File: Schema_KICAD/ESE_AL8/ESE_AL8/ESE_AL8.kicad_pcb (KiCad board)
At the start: 4 copper layers, 54 x 57 mm, 85 parts, among them IC1 MP1475SGJ-P, J1 CB1, J2 CB2, J3 LIDAR, J4 Moteur1, J5 Moteur2, J6 Batterie, J7 Conn_ST_STDC14, J8 ECRAN, SW1 SW_c/s, SW2 ON/OFF, U1 ADXL343, U2 BUxxSD5, U3 STM32G431CBUx, U4 ZXBM5210-SP, U5 ZXBM5210-SP, Y1 16MHz

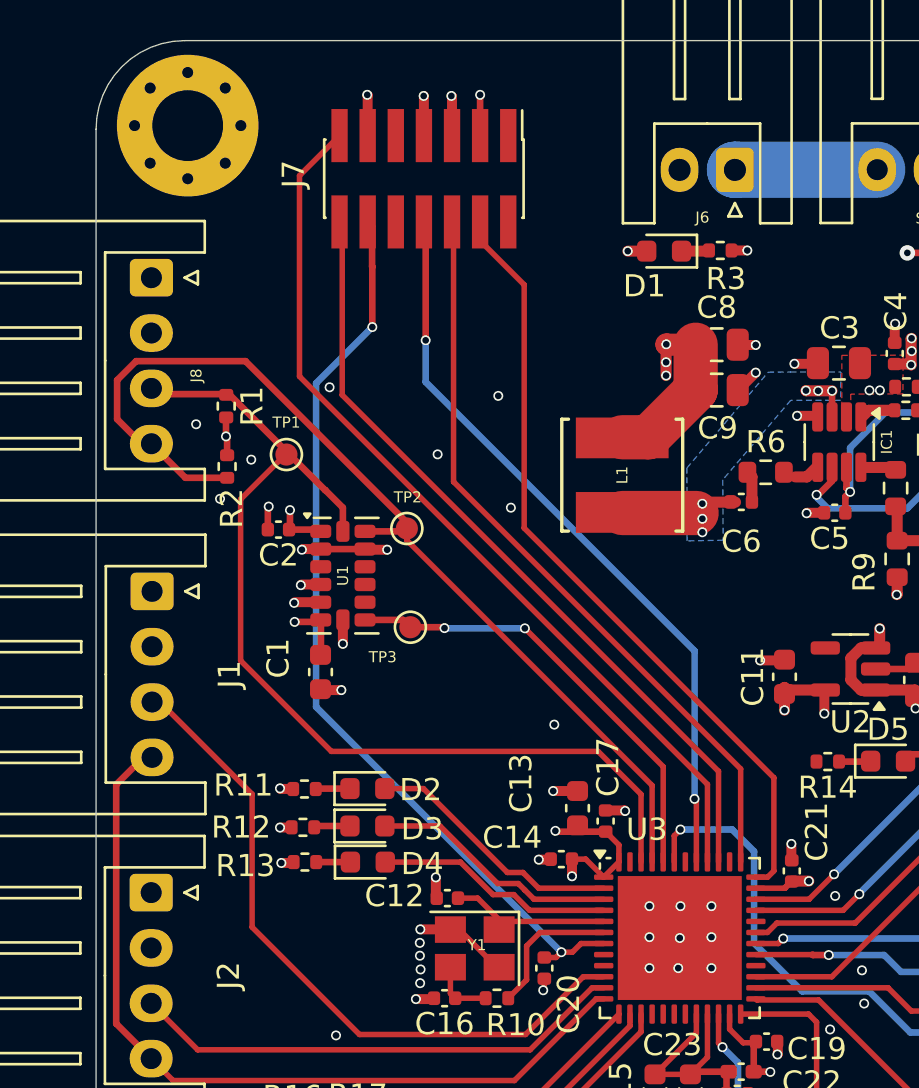
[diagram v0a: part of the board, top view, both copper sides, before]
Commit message: Commit midif pcb 23/10 0816
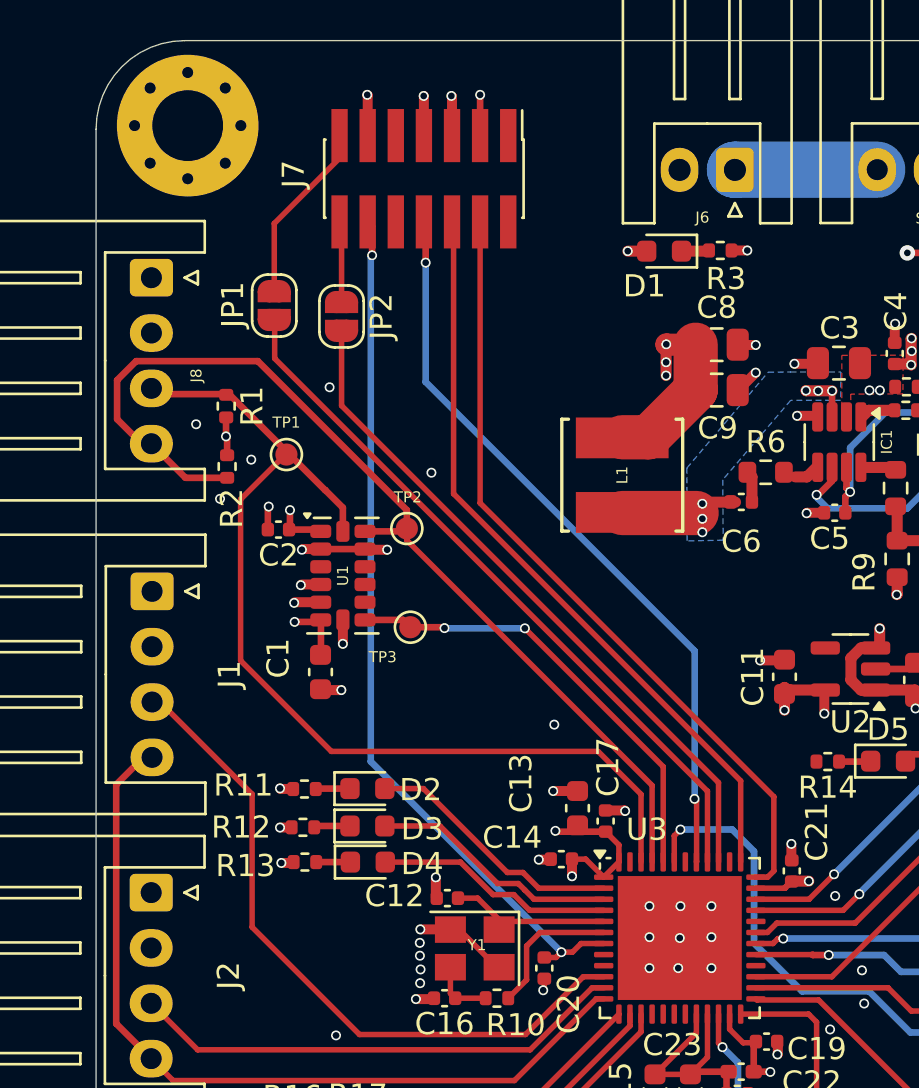
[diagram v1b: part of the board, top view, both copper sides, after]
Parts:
- added JP1: SolderJumper_2_Open, Jumper:SolderJumper-2_P1.3mm_Open_RoundedPad1.0x1.5mm, F.Cu at (138.1, 78.0)
- added JP2: SolderJumper_2_Open, Jumper:SolderJumper-2_P1.3mm_Open_RoundedPad1.0x1.5mm, F.Cu at (141.1, 78.5)
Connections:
- J7 pad 13: RX_SWD -> Net-(J7-VCP_RX)
- J7 pad 14: TX_SWD -> Net-(J7-VCP_TX)
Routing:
- net RX_SWD: track 41.2 -> 32.6 mm
- net Net-(J7-VCP_RX): track 0.00 -> 8.48 mm
- net TX_SWD: track 36.0 -> 31.1 mm
- net Net-(J7-VCP_TX): track 0.00 -> 3.66 mm
- net NRST: track 41.7 -> 39.6 mm
- net GND: vias 95 -> 93
